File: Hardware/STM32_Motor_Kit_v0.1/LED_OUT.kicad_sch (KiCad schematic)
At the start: 24 parts, among them Q7 MMUN2235LT1G, U15 SN74HC595DRG3

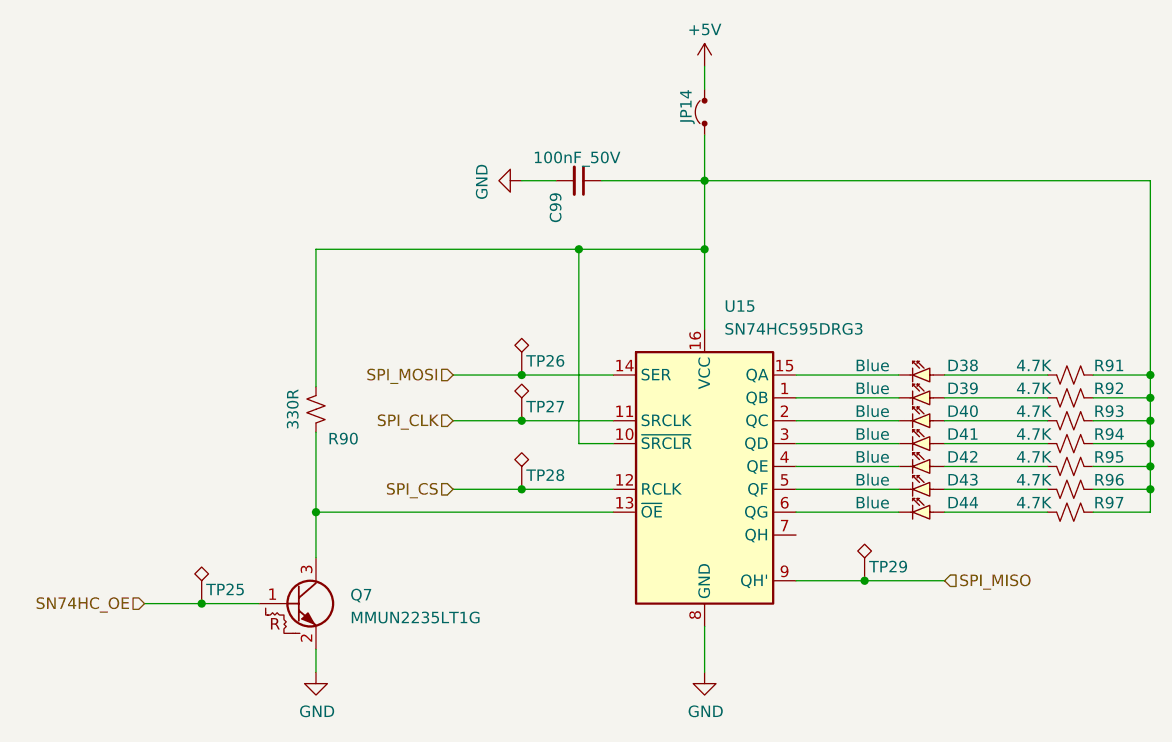
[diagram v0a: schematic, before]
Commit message: 12.01.2025
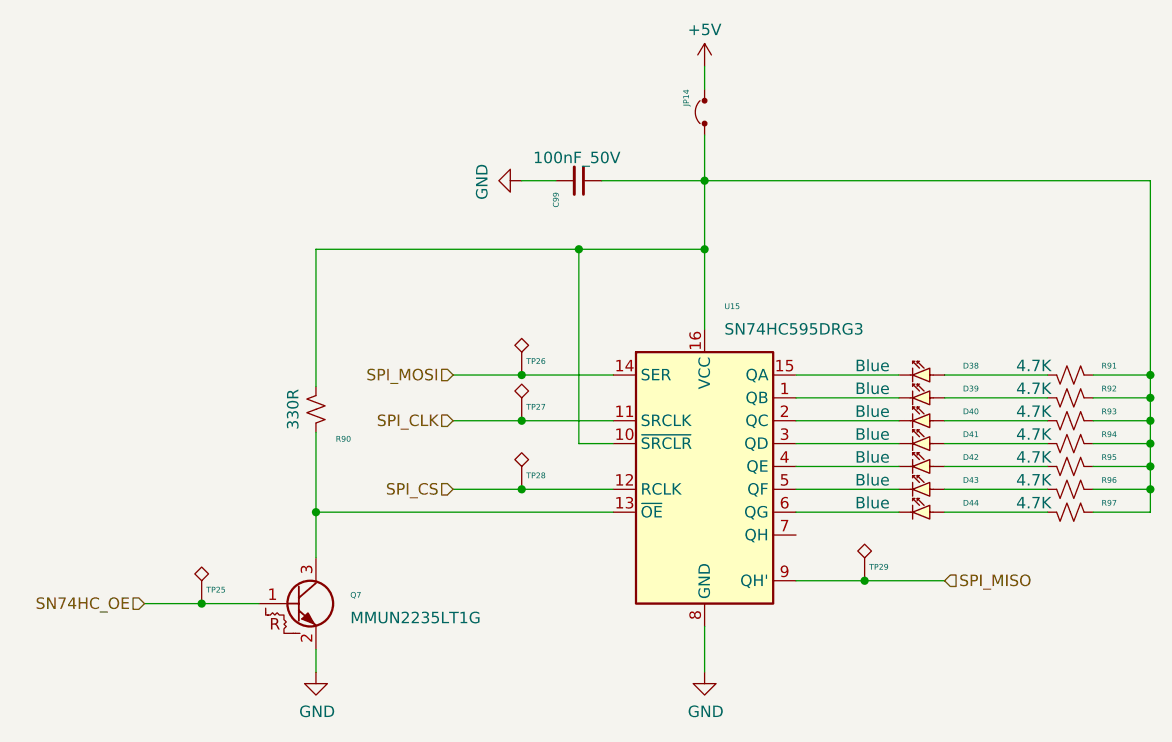
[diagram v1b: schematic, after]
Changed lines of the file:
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@@
 			(effects
 				(font
-					(size 1.27 1.27)
+					(face "Arial")
+					(size 0.635 0.635)
 				)
 				(hide yes)
@@
 			(effects
 				(font
-					(size 1.27 1.27)
+					(face "Arial")
+					(size 0.635 0.635)
 				)
 				(justify right)
@@
 			(effects
 				(font
-					(size 1.27 1.27)
+					(face "Arial")
+					(size 0.635 0.635)
 				)
 			)
@@
 			(effects
 				(font
-					(size 1.27 1.27)
+					(face "Arial")
+					(size 0.635 0.635)
 				)
 				(hide yes)
@@
 			(effects
 				(font
-					(size 1.27 1.27)
+					(face "Arial")
+					(size 0.635 0.635)
 				)
 				(hide yes)
@@
 			(effects
 				(font
-					(size 1.27 1.27)
+					(face "Arial")
+					(size 0.635 0.635)
 				)
 				(justify left)
@@
 			(effects
 				(font
-					(size 1.27 1.27)
+					(face "Arial")
+					(size 0.635 0.635)
 				)
 				(justify left)
@@
 			(effects
 				(font
-					(size 1.27 1.27)
+					(face "Arial")
+					(size 0.635 0.635)
 				)
 			)
@@
 			(effects
 				(font
-					(size 1.27 1.27)
+					(face "Arial")
+					(size 0.635 0.635)
 				)
 			)
@@
 			(effects
 				(font
-					(size 1.27 1.27)
+					(face "Arial")
+					(size 0.635 0.635)
 				)
 			)
@@
 			(effects
 				(font
-					(size 1.27 1.27)
+					(face "Arial")
+					(size 0.635 0.635)
 				)
 				(justify left)
@@
 			(effects
 				(font
-					(size 1.27 1.27)
+					(face "Arial")
+					(size 0.635 0.635)
 				)
 				(justify right)
@@
 			(effects
 				(font
-					(size 1.27 1.27)
+					(face "Arial")
+					(size 0.635 0.635)
 				)
 				(hide yes)
@@
 			(effects
 				(font
-					(size 1.27 1.27)
+					(face "Arial")
+					(size 0.635 0.635)
 				)
 			)
@@
 			(effects
 				(font
-					(size 1.27 1.27)
+					(face "Arial")
+					(size 0.635 0.635)
 				)
 			)
@@
 			(effects
 				(font
-					(size 1.27 1.27)
+					(face "Arial")
+					(size 0.635 0.635)
 				)
 				(justify left)
@@
 			(effects
 				(font
-					(size 1.27 1.27)
+					(face "Arial")
+					(size 0.635 0.635)
 				)
 				(justify right)
@@
 			(effects
 				(font
-					(size 1.27 1.27)
+					(face "Arial")
+					(size 0.635 0.635)
 				)
 				(justify right)
@@
 			(effects
 				(font
-					(size 1.27 1.27)
+					(face "Arial")
+					(size 0.635 0.635)
 				)
 			)
@@
 			(effects
 				(font
-					(size 1.27 1.27)
+					(face "Arial")
+					(size 0.635 0.635)
 				)
 				(justify right)
@@
 			(effects
 				(font
-					(size 1.27 1.27)
+					(face "Arial")
+					(size 0.635 0.635)
 				)
 				(justify right)
@@
 			(effects
 				(font
-					(size 1.27 1.27)
+					(face "Arial")
+					(size 0.635 0.635)
 				)
 				(justify left)
@@
 			(effects
 				(font
-					(size 1.27 1.27)
+					(face "Arial")
+					(size 0.635 0.635)
 				)
 				(justify right)
@@
 			(effects
 				(font
-					(size 1.27 1.27)
+					(face "Arial")
+					(size 0.635 0.635)
 				)
 				(justify right)
@@
 			(effects
 				(font
-					(size 1.27 1.27)
+					(face "Arial")
+					(size 0.635 0.635)
 				)
 				(justify left)
@@
 			(effects
 				(font
-					(size 1.27 1.27)
+					(face "Arial")
+					(size 0.635 0.635)
 				)
 			)
@@
 			(effects
 				(font
-					(size 1.27 1.27)
+					(face "Arial")
+					(size 0.635 0.635)
 				)
 				(justify left)
@@
 			(effects
 				(font
-					(size 1.27 1.27)
+					(face "Arial")
+					(size 0.635 0.635)
 				)
 				(justify left)

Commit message: Şema üzerinde değişiklikler devam ediyor
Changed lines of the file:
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@@
 (kicad_sch
-	(version 20231120)
+	(version 20250114)
 	(generator "eeschema")
-	(generator_version "8.0")
+	(generator_version "9.0")
 	(paper "A4")
 	(junction
@@
 		(shape input)
 		(at 74.93 97.79 180)
-		(fields_autoplaced yes)
 		(effects
 			(font
@@
 		(shape input)
 		(at 109.22 85.09 180)
-		(fields_autoplaced yes)
 		(effects
 			(font
@@
 		(shape input)
 		(at 109.22 72.39 180)
-		(fields_autoplaced yes)
 		(effects
 			(font
@@
 		(shape input)
 		(at 163.83 95.25 0)
-		(fields_autoplaced yes)
 		(effects
 			(font
@@
 		(shape input)
 		(at 109.22 77.47 180)
-		(fields_autoplaced yes)
 		(effects
 			(font
